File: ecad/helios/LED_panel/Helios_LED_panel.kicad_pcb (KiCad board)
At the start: 2 copper layers, 100 x 100 mm, 42 parts

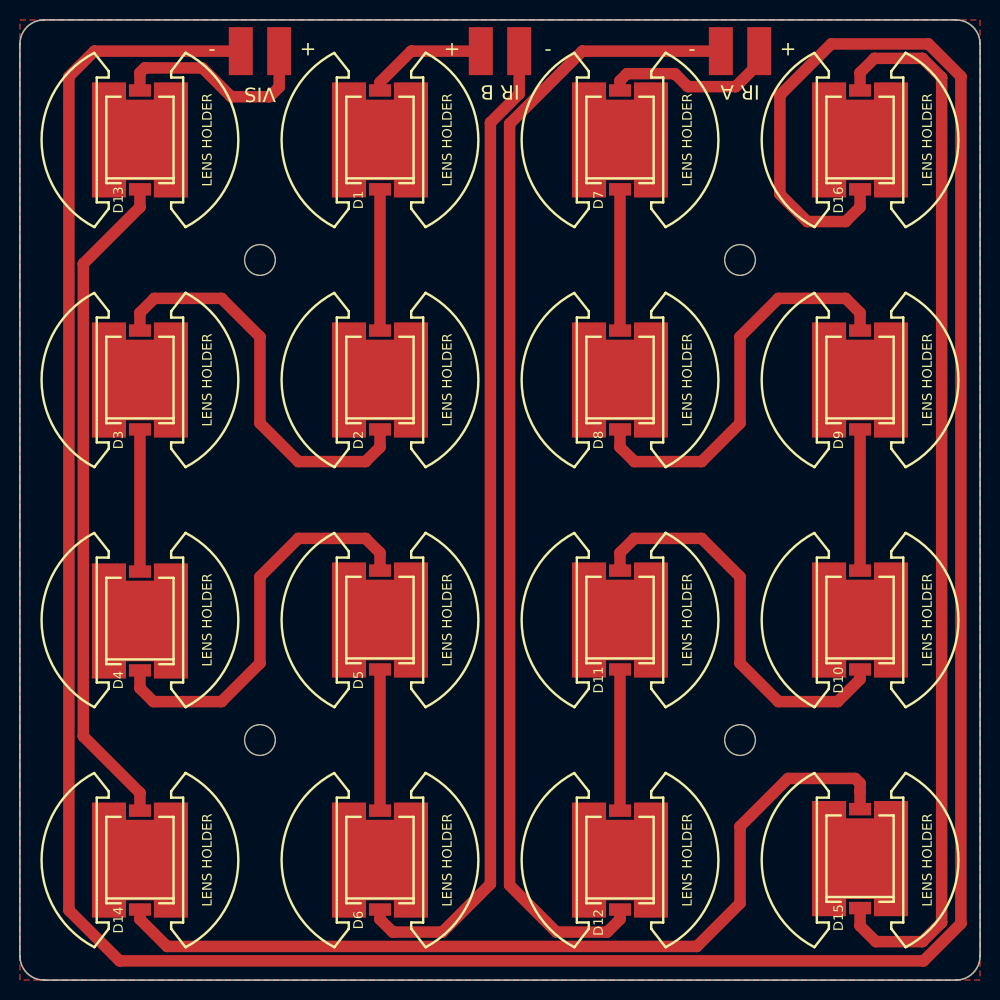
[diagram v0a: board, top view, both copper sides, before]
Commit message: wip
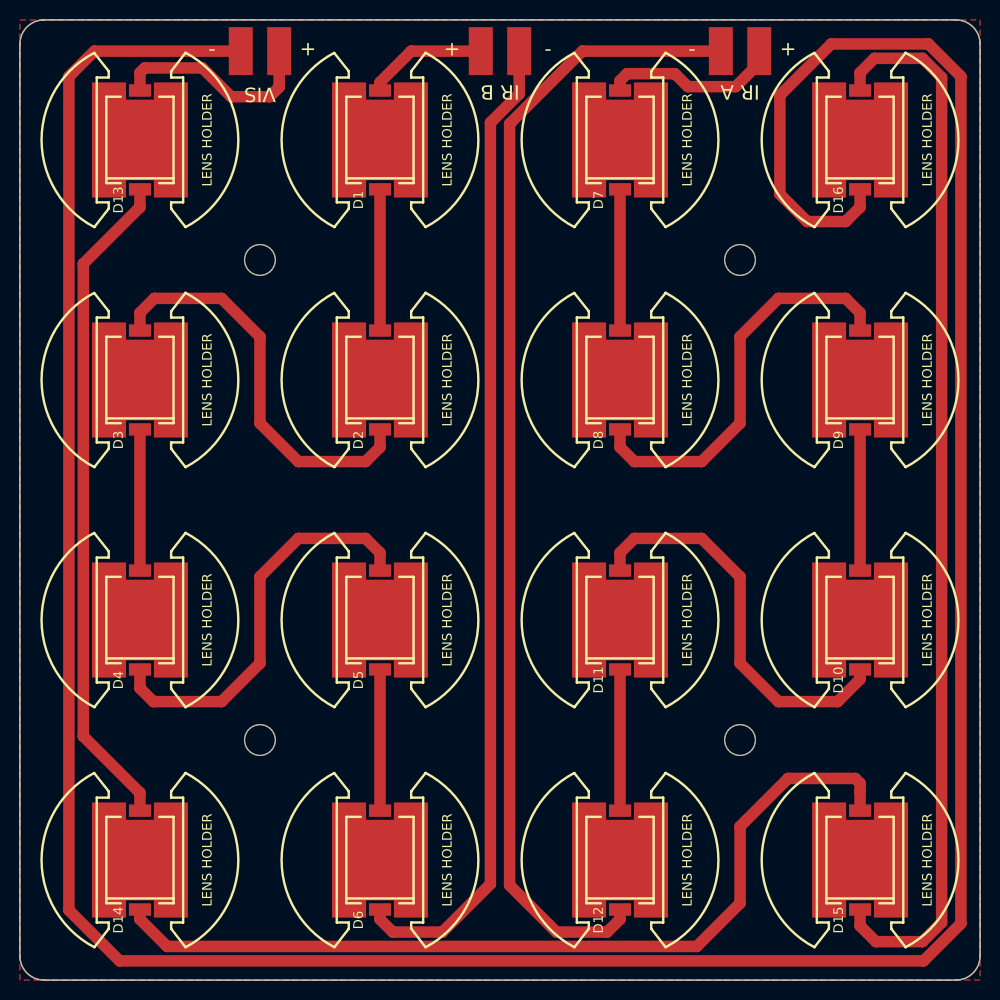
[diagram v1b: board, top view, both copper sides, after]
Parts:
- D1, D10, D11, D12, D2, D3, D4, D5, D6, D7, D8, D9: value NIR 850nm 3W -> SFH 4235-Z
- D13, D14, D15, D16: value White 4000K 3W -> LSW W5SM
- moved D15 0.15 mm to (207.5, 147.5), turned to 180 degrees
- moved D4 0.10 mm to (132.5, 122.5), turned to 180 degrees
- turned D1 to 180 degrees
- turned D10 to 180 degrees
- turned D11 to 180 degrees
- turned D12 to 180 degrees
- turned D13 to 180 degrees
- turned D14 to 180 degrees
- turned D16 to 180 degrees
- turned D2 to 180 degrees
- turned D3 to 180 degrees
- turned D5 to 180 degrees
- turned D6 to 180 degrees
- turned D7 to 180 degrees
- turned D8 to 180 degrees
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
